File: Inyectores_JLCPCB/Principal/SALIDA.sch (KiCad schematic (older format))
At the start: 24 parts, among them J5 INY2, J6 INY1, J7 INY4, J8 INY3, Q1 IRF540N, Q2 IRF540N, Q3 IRF540N, Q4 IRF540N, U3 PC817_INY1, U4 PC817_INY2, U5 PC817_INY3, U6 PC817_INY4

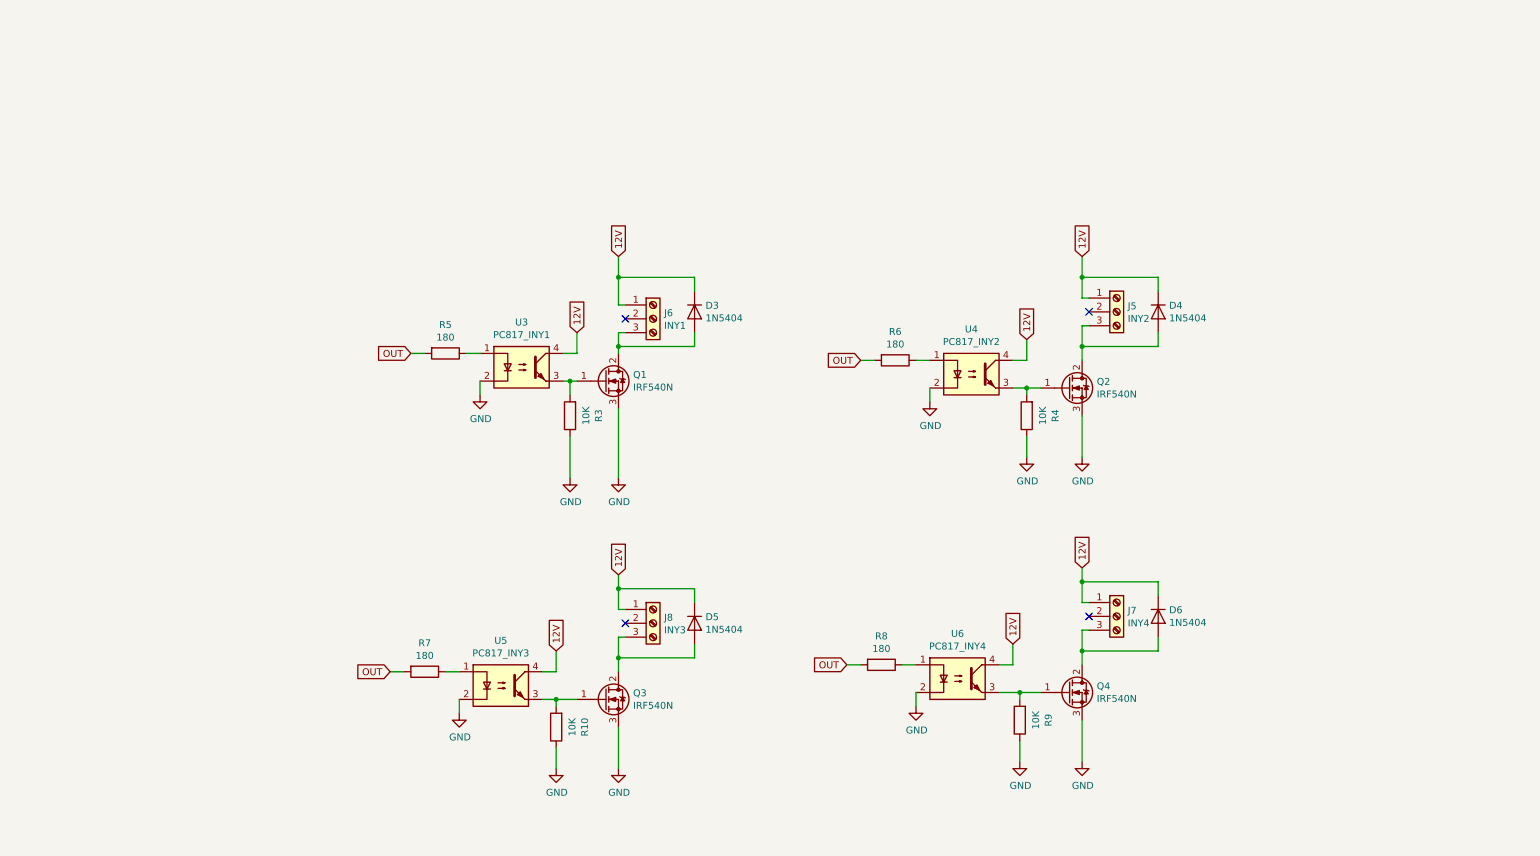
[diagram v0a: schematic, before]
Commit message: -
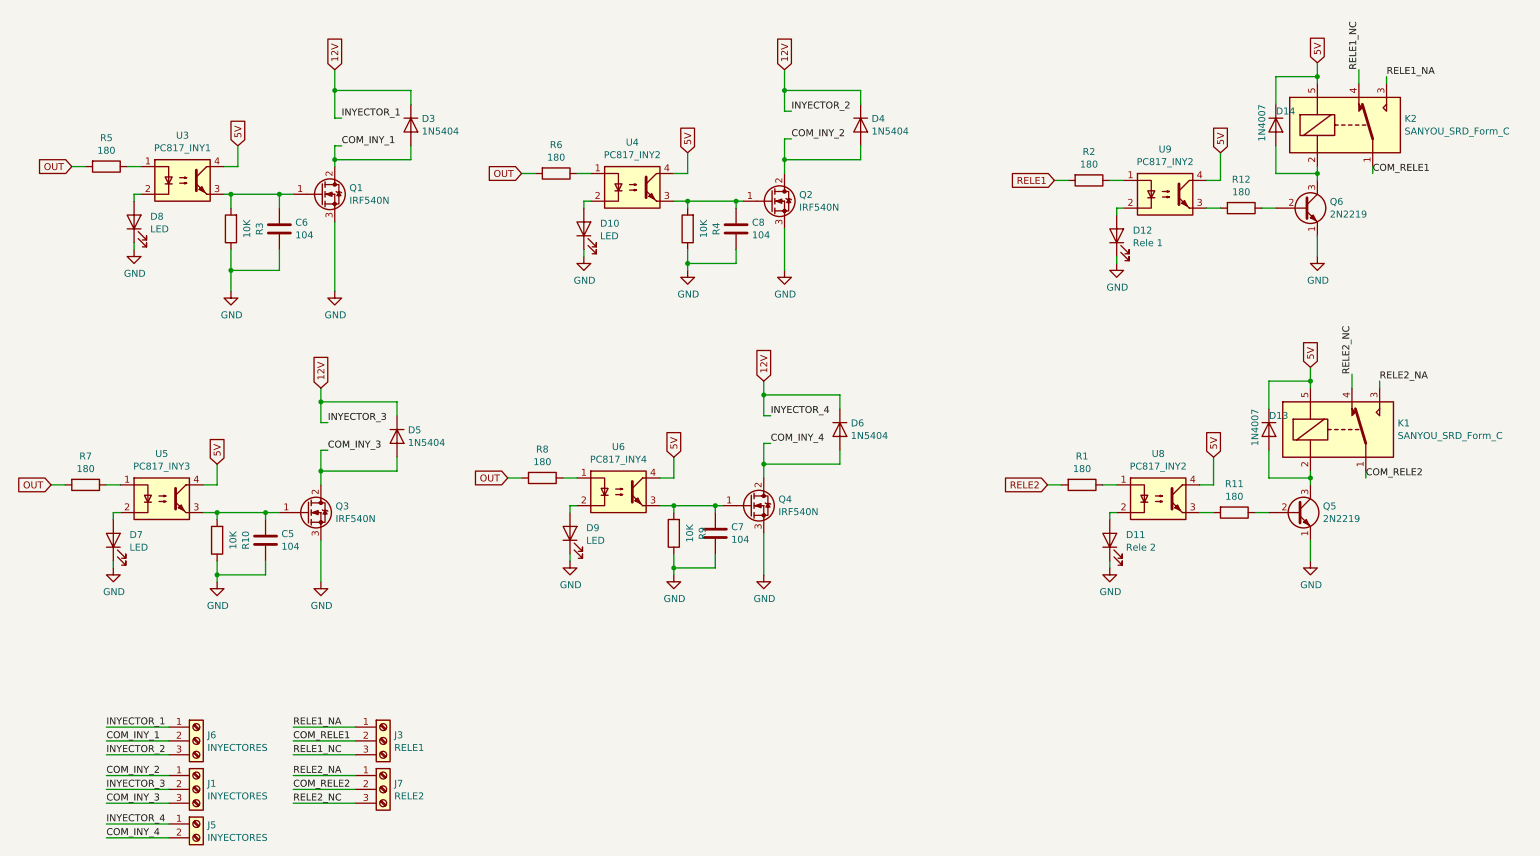
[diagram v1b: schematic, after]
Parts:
- removed J5: INY2, BorneraTornillos:bornera_tornillos_1x03, symbol Connector:Screw_Terminal_01x03
- removed J8: INY3, BorneraTornillos:bornera_tornillos_1x03, symbol Connector:Screw_Terminal_01x03
- added C5, C6, C7, C8: 104, Capacitor_THT:C_Disc_D3.4mm_W2.1mm_P2.50mm, symbol Device:C
- added D10, D7, D8, D9: LED, LED_SMD:LED_0805_2012Metric, symbol Device:LED
- added D11: Rele 2, LED_SMD:LED_0805_2012Metric, symbol Device:LED
- added D12: Rele 1, LED_SMD:LED_0805_2012Metric, symbol Device:LED
- added D13, D14: 1N4007, Diode_THT:D_DO-41_SOD81_P10.16mm_Horizontal, symbol Diode:1N4007
- added J1: INYECTORES, BorneraTornillos:TerminalBlock_Phoenix_PT-1,5-3-5.0-H_1x03_P5.00mm_Horizontal, symbol Connector:Screw_Terminal_01x03
- added J3: RELE1, BorneraTornillos:TerminalBlock_Phoenix_PT-1,5-3-5.0-H_1x03_P5.00mm_Horizontal, symbol Connector:Screw_Terminal_01x03
- added J5: INYECTORES, BorneraTornillos:TerminalBlock_Phoenix_PT-1,5-2-5.0-H_1x02_P5.00mm_Horizontal, symbol Connector:Screw_Terminal_01x02
- added K1, K2: SANYOU_SRD_Form_C, Relay_THT:Relay_SPDT_SANYOU_SRD_Series_Form_C, symbol Relay:SANYOU_SRD_Form_C
- added Q5, Q6: 2N2219, Package_TO_SOT_THT:TO-92_Inline, symbol Transistor_BJT:2N2219
- added R1, R11, R12, R2: 180, Resistor_THT:R_Axial_DIN0207_L6.3mm_D2.5mm_P10.16mm_Horizontal, symbol Device:R
- added U8, U9: PC817_INY2, Package_DIP:DIP-4_W7.62mm_LongPads, symbol Isolator:PC817
- J6: value INY1 -> INYECTORES; footprint BorneraTornillos:bornera_tornillos_1x03 -> BorneraTornillos:TerminalBlock_Phoenix_PT-1,5-3-5.0-H_1x03_P5.00mm_Horizontal
- J7: value INY4 -> RELE2; footprint BorneraTornillos:bornera_tornillos_1x03 -> BorneraTornillos:TerminalBlock_Phoenix_PT-1,5-3-5.0-H_1x03_P5.00mm_Horizontal
- Q1, Q2, Q3, Q4: footprint Package_TO_SOT_THT:TO-220-3_Horizontal_TabDown -> Package_TO_SOT_THT:TO-220-3_Vertical
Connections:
- net 12V: now also J6.3 (Pin_3), J1.2 (Pin_2), J5.1 (Pin_1); no longer J7.1 (Pin_1), U3.4, U4.4, U5.4, U6.4
- net GND: now also C5.2, C6.2, C7.2, C8.2, D10.1 (K), D11.1 (K), D12.1 (K), D7.1 (K), D8.1 (K), D9.1 (K), Q5.1 (E), Q6.1 (E); no longer U3.2, U4.2, U5.2, U6.2
- net at Q1.1 (G), R3.2, U3.3: now also C6.1
- net COM_INY_1: now reaches D3.2 (A), Q1.2 (D)
- net COM_INY_1: now also J6.2 (Pin_2); no longer J6.3 (Pin_3)
- net at Q3.1 (G), R10.2, U5.3: now also C5.1
- net COM_INY_3: now reaches D5.2 (A), Q3.2 (D)
- net COM_INY_3: now also J1.3 (Pin_3)
- net at Q2.1 (G), R4.2, U4.3: now also C8.1
- net COM_INY_2: now reaches D4.2 (A), Q2.2 (D)
- net COM_INY_2: now also J1.1 (Pin_1)
- net at Q4.1 (G), R9.2, U6.3: now also C7.1
- net COM_INY_4: now reaches D6.2 (A), Q4.2 (D)
- net COM_INY_4: now also J5.2 (Pin_2); no longer J7.3 (Pin_3)
- net COM_RELE2: now reaches J7.2 (Pin_2)
- net COM_RELE2: now also K1.1
- new net: D8.2 (A), U3.2
- new net: D7.2 (A), U5.2
- new net: D10.2 (A), U4.2
- new net: D9.2 (A), U6.2
- new net: R2.1, U9.1
- new net: D12.2 (A), U9.2
- new net: R12.2, U9.3
- new net: Q6.2 (B), R12.1
- new net: D14.2 (A), K2.2, Q6.3 (C)
- new net: R1.1, U8.1
- new net: D11.2 (A), U8.2
- new net: R11.2, U8.3
- new net: Q5.2 (B), R11.1
- new net: D13.2 (A), K1.2, Q5.3 (C)
- new net 5V: D13.1 (K), D14.1 (K), K1.5, K2.5, U3.4, U4.4, U5.4, U6.4, U8.4, U9.4
- new net COM_RELE1: J3.2 (Pin_2), K2.1
- new net RELE1: R2.2
- new net RELE1_NA: J3.1 (Pin_1), K2.3
- new net RELE1_NC: J3.3 (Pin_3), K2.4
- new net RELE2: R1.2
- new net RELE2_NA: J7.1 (Pin_1), K1.3
- new net RELE2_NC: J7.3 (Pin_3), K1.4
- no-connect marks 4 -> 0
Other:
- moved on the sheet: D3, D4, D5, D6, J6, Q1, Q2, Q3, Q4, R10, R3, R4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
